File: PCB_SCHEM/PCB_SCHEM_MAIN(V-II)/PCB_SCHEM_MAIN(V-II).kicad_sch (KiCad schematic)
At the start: 2 parts, among them U1 RP2040, U2 TPS61291DRVR

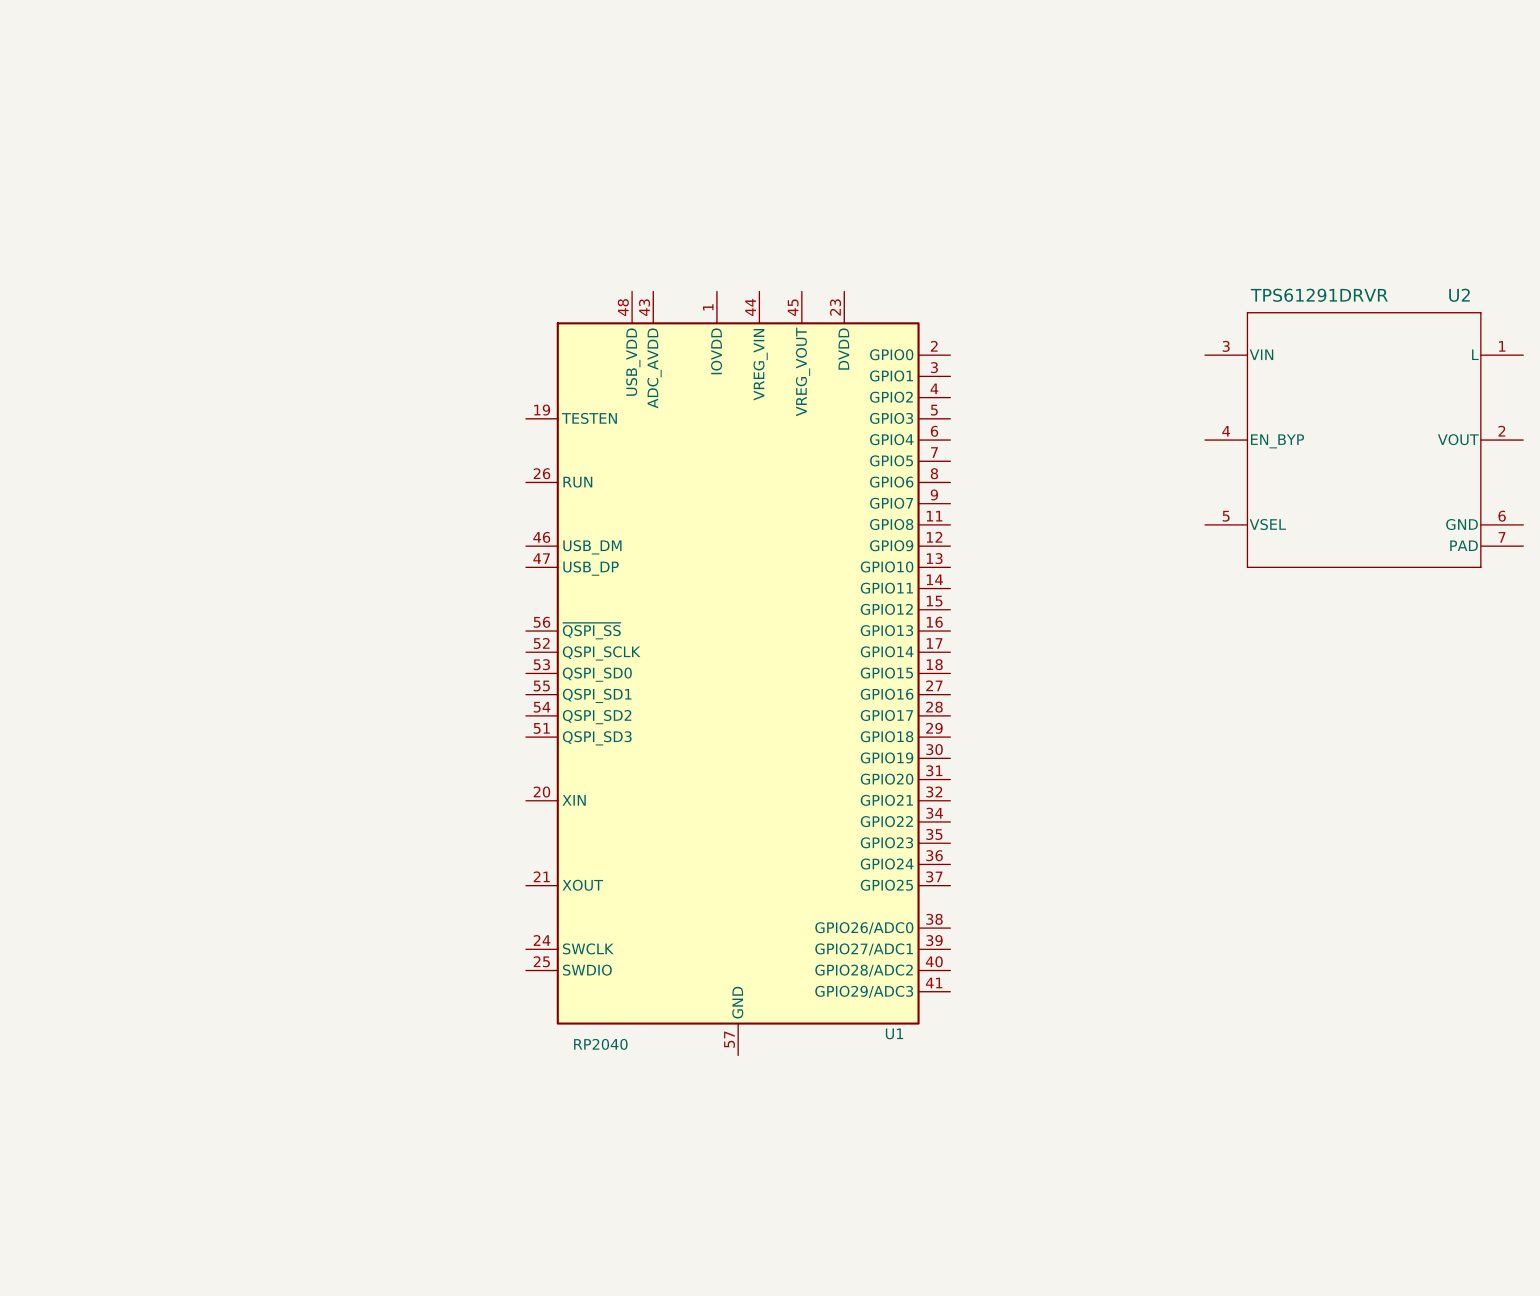
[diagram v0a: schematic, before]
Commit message: Added all the IC's, the main framework of the PCB done. Minor wiring and final touches left
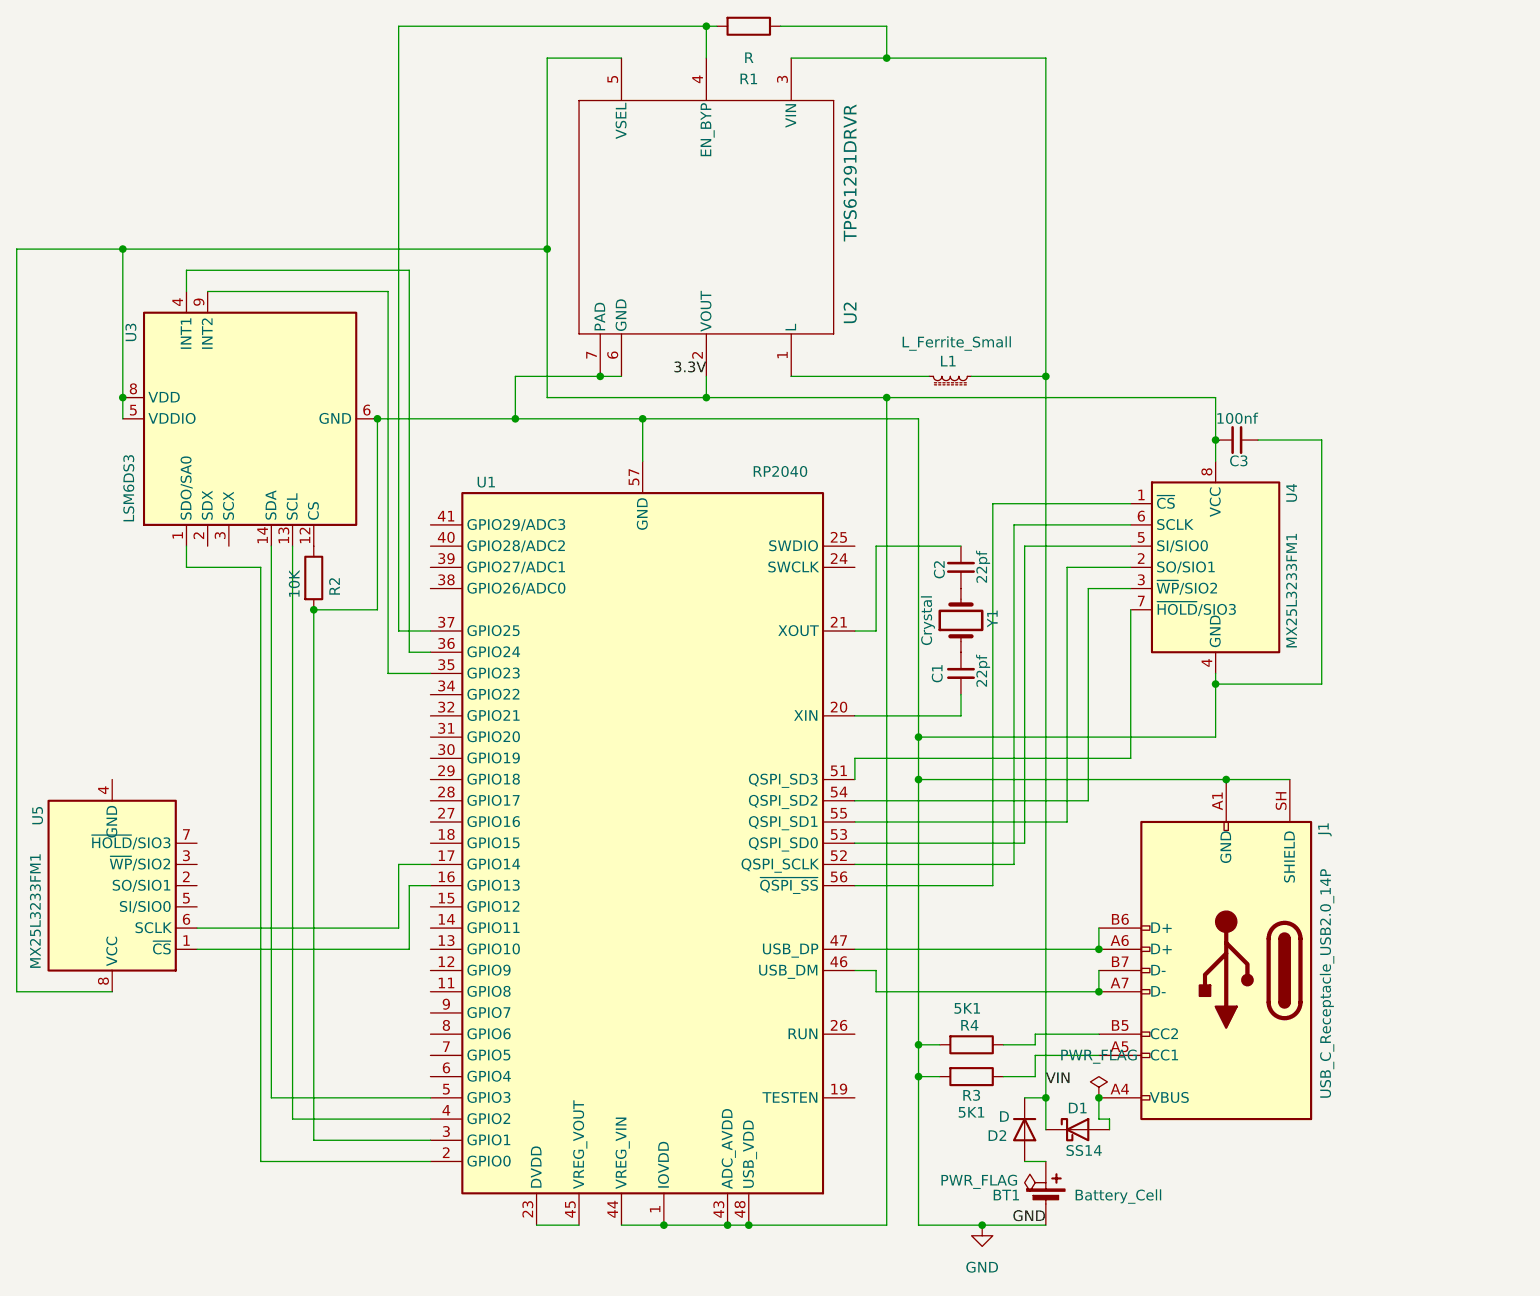
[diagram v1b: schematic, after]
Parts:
- added BT1: Battery_Cell, Package_SON:Texas_DRC0010J_ThermalVias, symbol Device:Battery_Cell
- added C1, C2: 22pf, Package_SO:SOIC-8_3.9x4.9mm_P1.27mm, symbol Device:C_Small
- added C3: 100nf, Package_SO:SOIC-8_3.9x4.9mm_P1.27mm, symbol Device:C_Small
- added D1: SS14, Diode_SMD:D_SMA, symbol Diode:SS14
- added D2: D, Diode_SMD:D_SMA, symbol Device:D
- added J1: USB_C_Receptacle_USB2.0_14P, Package_DFN_QFN:WDFN-10-1EP_3x3mm_P0.5mm_EP1.8x2.5mm, symbol Connector:USB_C_Receptacle_USB2.0_14P
- added L1: L_Ferrite_Small, Package_BGA:BGA-624_21x21mm_Layout25x25_P0.8mm, symbol Device:L_Ferrite_Small
- added R1: R, Package_DIP:DIP-8_W7.62mm, symbol Device:R
- added R2: 10K, Package_DIP:DIP-8_W7.62mm, symbol Device:R
- added R3, R4: 5K1, Package_DIP:DIP-8_W7.62mm, symbol Device:R
- added U3: LSM6DS3, Package_LGA:LGA-14_3x2.5mm_P0.5mm_LayoutBorder3x4y, symbol Sensor_Motion:LSM6DS3
- added U4, U5: MX25L3233FM1, Package_SO:JEITA_SOIC-8_3.9x4.9mm_P1.27mm, symbol Memory_Flash:MX25L3233FM1
- added Y1: Crystal, Package_SO:JEITA_SOIC-8_3.9x4.9mm_P1.27mm, symbol Device:Crystal
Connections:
- net at U2.1 (L): now also L1.2
- net 3.3V: now reaches U2.2 (VOUT)
- net 3.3V: now also U1.1 (IOVDD), U1.10 (IOVDD), U1.22 (IOVDD), U1.33 (IOVDD), U1.42 (IOVDD), U1.43 (ADC_AVDD), U1.44 (VREG_VIN), U1.48 (USB_VDD), U1.49 (IOVDD), U2.5 (VSEL), C3.2, U3.5 (VDDIO), U3.8 (VDD), U4.8 (VCC), U5.8 (VCC)
- net VIN: now reaches U2.3 (VIN)
- net VIN: now also D1.1 (K), D2.1 (K), L1.1, R1.1
- net at U2.4 (EN_BYP): now also U1.37 (GPIO25), R1.2
- net GND: now reaches U2.6 (GND)
- net GND: now also U1.3 (GPIO1), U1.57 (GND), U2.7 (PAD), BT1.2 (-), C3.1, J1.A1 (GND), J1.A12 (GND), J1.B1 (GND), J1.B12 (GND), J1.SH (SHIELD), R2.2, R3.2, R4.2, U3.6 (GND), U3.7 (GND), U4.4 (GND)
- net at U1.16 (GPIO13): now also U5.1 (~{CS})
- net at U1.17 (GPIO14): now also U5.6 (SCLK)
- net at U1.2 (GPIO0): now also U3.1 (SDO/SA0)
- net at U1.20 (XIN): now also C1.1
- net at U1.21 (XOUT): now also C2.2
- net at U1.23 (DVDD), U1.50 (DVDD): now also U1.45 (VREG_VOUT)
- net at U1.35 (GPIO23): now also U3.9 (INT2)
- net at U1.36 (GPIO24): now also U3.4 (INT1)
- net at U1.4 (GPIO2): now also U3.13 (SCL)
- net at U1.46 (USB_DM): now also J1.A7 (D-), J1.B7 (D-)
- net at U1.47 (USB_DP): now also J1.A6 (D+), J1.B6 (D+)
- net at U1.5 (GPIO3): now also U3.14 (SDA)
- net at U1.51 (QSPI_SD3): now also U4.7 (~{HOLD}/SIO3)
- net at U1.52 (QSPI_SCLK): now also U4.6 (SCLK)
- net at U1.53 (QSPI_SD0): now also U4.5 (SI/SIO0)
- net at U1.54 (QSPI_SD2): now also U4.3 (~{WP}/SIO2)
- net at U1.55 (QSPI_SD1): now also U4.2 (SO/SIO1)
- net at U1.56 (~{QSPI_SS}): now also U4.1 (~{CS})
- new net: J1.A5 (CC1), R3.1
- new net: D1.2 (A), J1.A4 (VBUS), J1.A9 (VBUS), J1.B4 (VBUS), J1.B9 (VBUS)
- new net: J1.B5 (CC2), R4.1
- new net: R2.1, U3.12 (CS)
- new net: C1.2, Y1.1
- new net: BT1.1 (+), D2.2 (A)
- new net: C2.1, Y1.2
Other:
- moved on the sheet: U1, U2
